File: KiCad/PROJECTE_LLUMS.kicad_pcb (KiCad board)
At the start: 2 copper layers, 138.1 x 86.1 mm, 62 parts, among them J1 CONNECTOR_MOTOR, J10 Conn_01x02_Pin, J2 DE9_Pins_MountingHoles, J3 Conn_01x05, J4 Conn_01x02_Pin, J5 DE9_Pins_MountingHoles, J6 Conn_01x02_Pin, J7 Conn_01x02_Pin, J8 Conn_01x02_Pin, J9 Conn_01x02_Pin, K1 Fujitsu_FTR-LYAA005x, Q2 IRLZ44N, Q3 IRLZ44N, Q4 IRLZ44N, Q5 IRLZ44N, Q6 IRLZ44N, Q7 IRLZ44N, SW1 SW_Push, SW2 SW_Push, SW3 SW_Push, SW4 SW_Push, SW5 SW_Push, SW6 SW_Push, U1 BH1750FVI-TR, U4 MCP2551-I-SN, U5 LM2596S-5, U6 LM1117MP-3.3, U7 PIC24HJ128GP502, Y1 8MHz

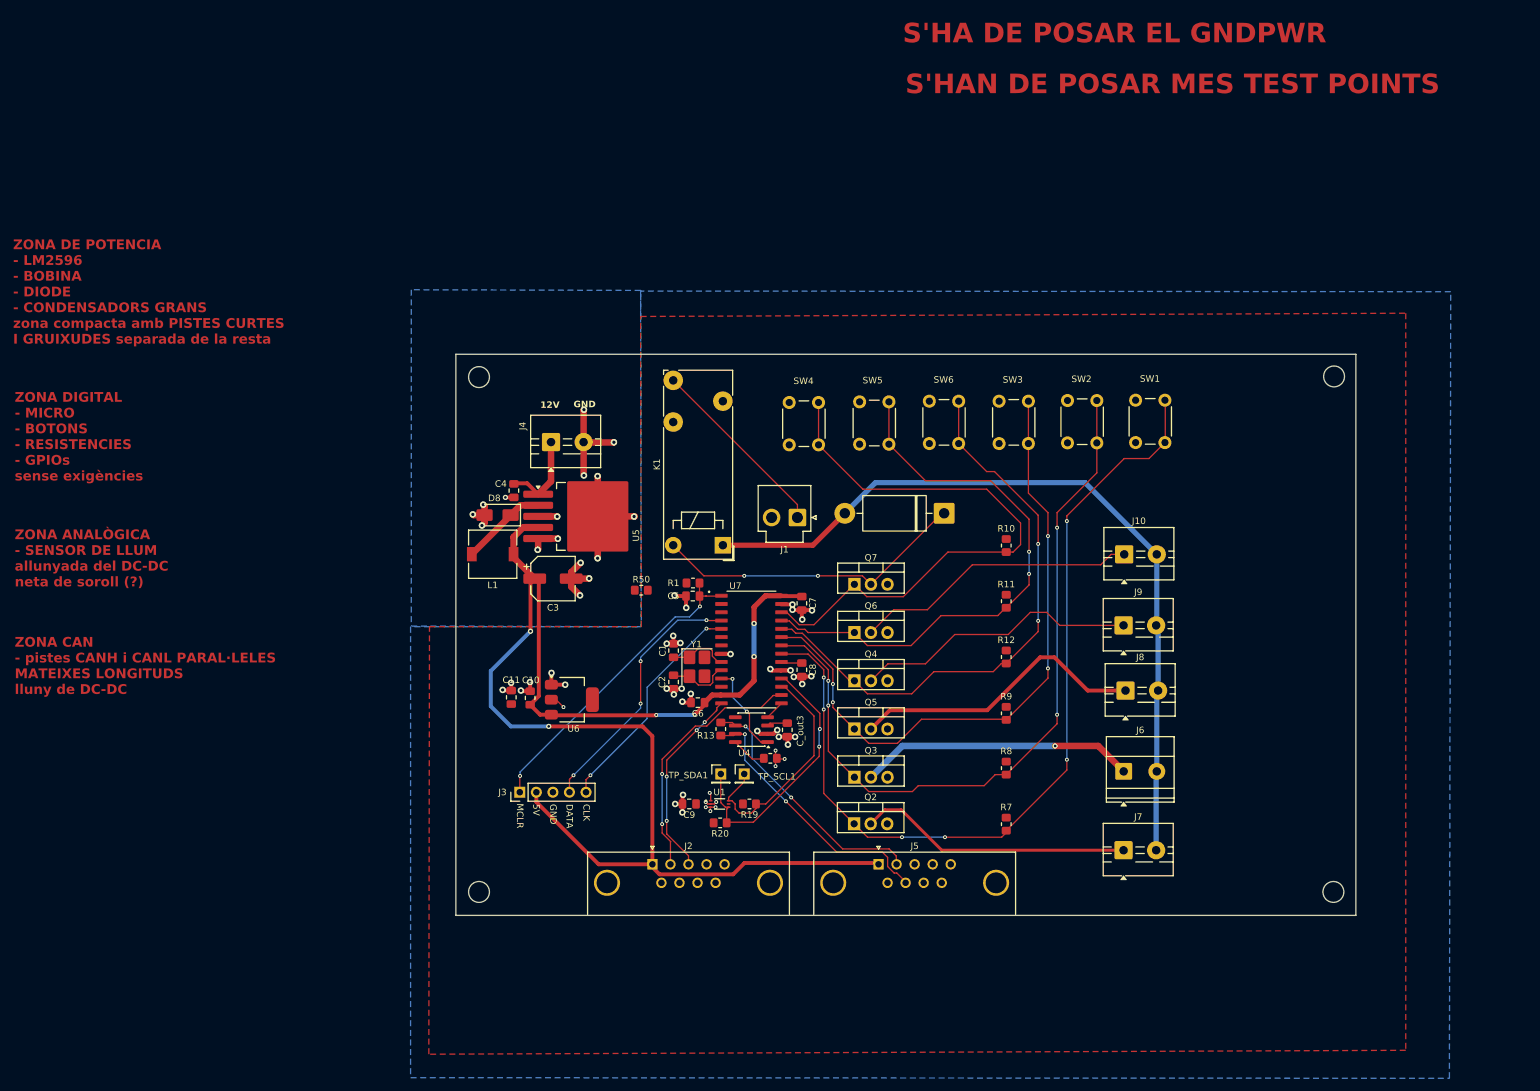
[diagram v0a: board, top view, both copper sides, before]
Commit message: correccions manel
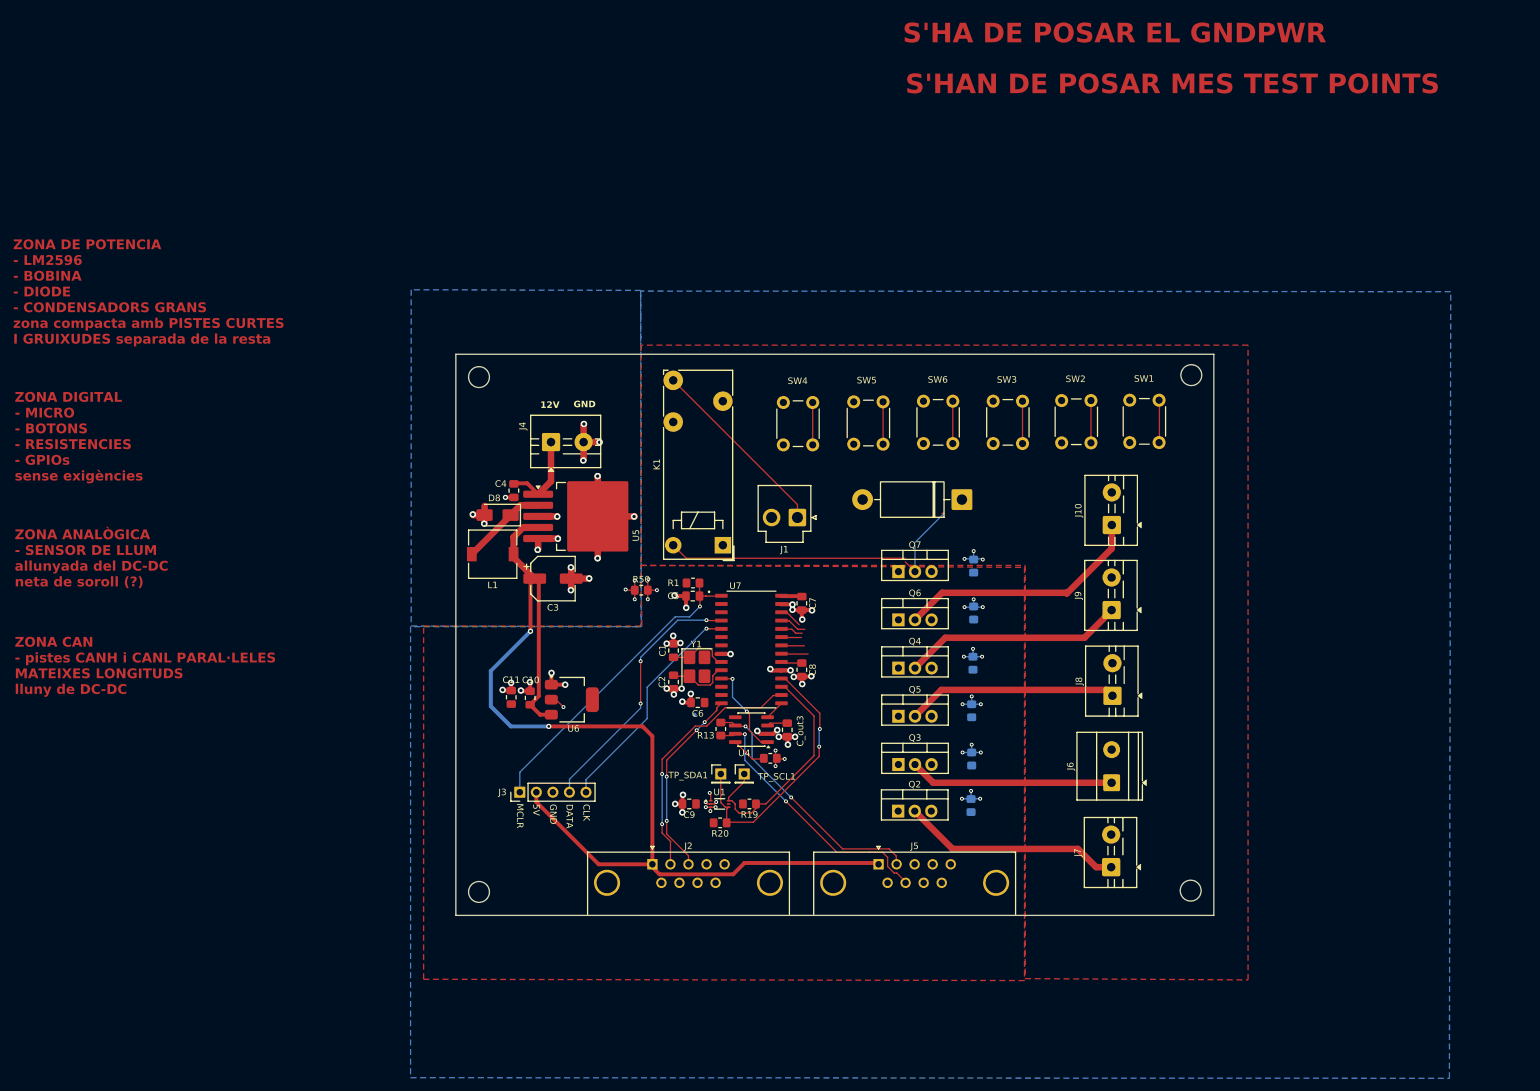
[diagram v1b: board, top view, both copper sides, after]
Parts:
- R10, R11, R12, R7, R8, R9: moved to B.Cu
- moved REF** 21.9 mm to (199.2, 117.0)
- moved REF** 21.9 mm to (199.3, 37.9)
- moved Q4 7.04 mm to (154.4, 82.8)
- moved Q5 7.04 mm to (154.4, 90.2)
- moved Q6 7.04 mm to (154.4, 75.5)
- moved Q7 7.04 mm to (154.4, 68.0)
- moved Q3 7.04 mm to (154.4, 97.7)
- moved Q2 7.04 mm to (154.3, 104.8)
- moved R7 6.11 mm to (165.5, 104.0)
- moved R10 5.91 mm to (165.9, 67.2)
- moved R8 5.48 mm to (165.6, 96.8)
- moved R9 5.32 mm to (165.6, 89.4)
- moved R11 5.31 mm to (165.9, 74.4)
- moved R12 5.19 mm to (165.8, 82.1)
- moved J10 4.88 mm to (187.1, 60.9), turned to 90 degrees
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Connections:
- C6 pad 1: +5V -> +3V3
- C7 pad 1: +5V -> +3V3
- U7 pad 13: +5V -> +3V3
- U7 pad 28: +5V -> +3V3
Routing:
- net CARRETERA: track 136.3 -> 10.7 mm, vias 6 -> 0
- net +12V: track 120.8 -> 0.00 mm
- net ENCREUAMENT: track 115.4 -> 10.1 mm, vias 4 -> 0
- net DIURNA: track 99.1 -> 9.63 mm, vias 4 -> 0
- net NETEJA-FARS: track 90.0 -> 10.1 mm
- net INTERM. ESQ: track 89.5 -> 10.0 mm, vias 2 -> 0
- net INTERM. DRT: track 86.7 -> 10.7 mm, vias 2 -> 0
- net +5V: track 217.4 -> 164.6 mm, vias 6 -> 2
- net +3V3: track 4.30 -> 31.9 mm, vias 2 -> 20
- net /llums/A_LED4: track 45.7 -> 32.4 mm
- net /llums/A_LED2: track 42.4 -> 31.3 mm, vias 1 -> 0
- net /llums/A_LED5: track 43.9 -> 33.9 mm
- net /llums/A_LED3: track 42.3 -> 33.7 mm
- net GNDPWR: track 56.3 -> 50.2 mm, vias 15 -> 18
- net /llums/A_LED6: track 43.8 -> 38.4 mm
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- added copper zone on F.Cu, net +12V
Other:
- board size 138.1 x 86.1 mm -> 116.3 x 86.1 mm
